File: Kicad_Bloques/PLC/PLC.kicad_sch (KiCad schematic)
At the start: 3 parts, among them J1 Conn_01x18_Socket, J2 Conn_01x18_Socket, U1 ESP32-S3-WROOM-1

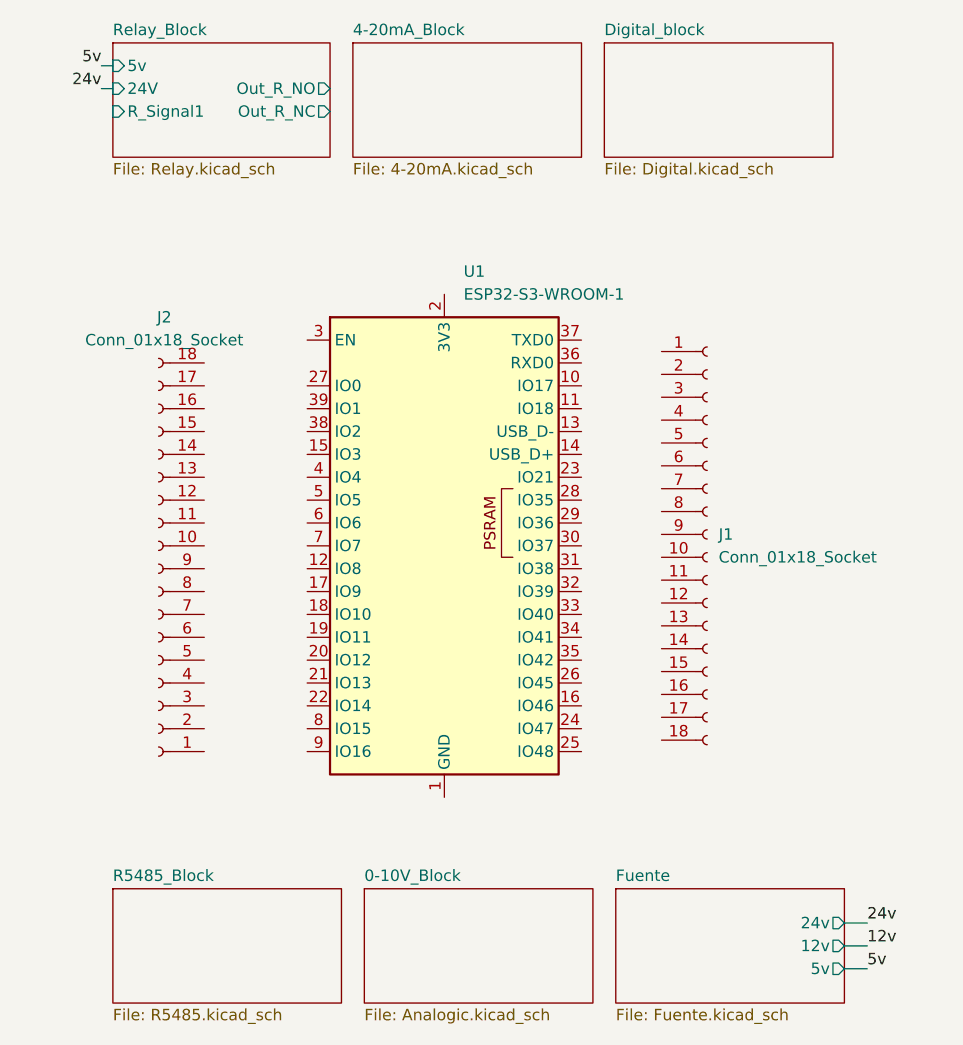
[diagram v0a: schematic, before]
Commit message: Actualizacion Bloques e Investigacion
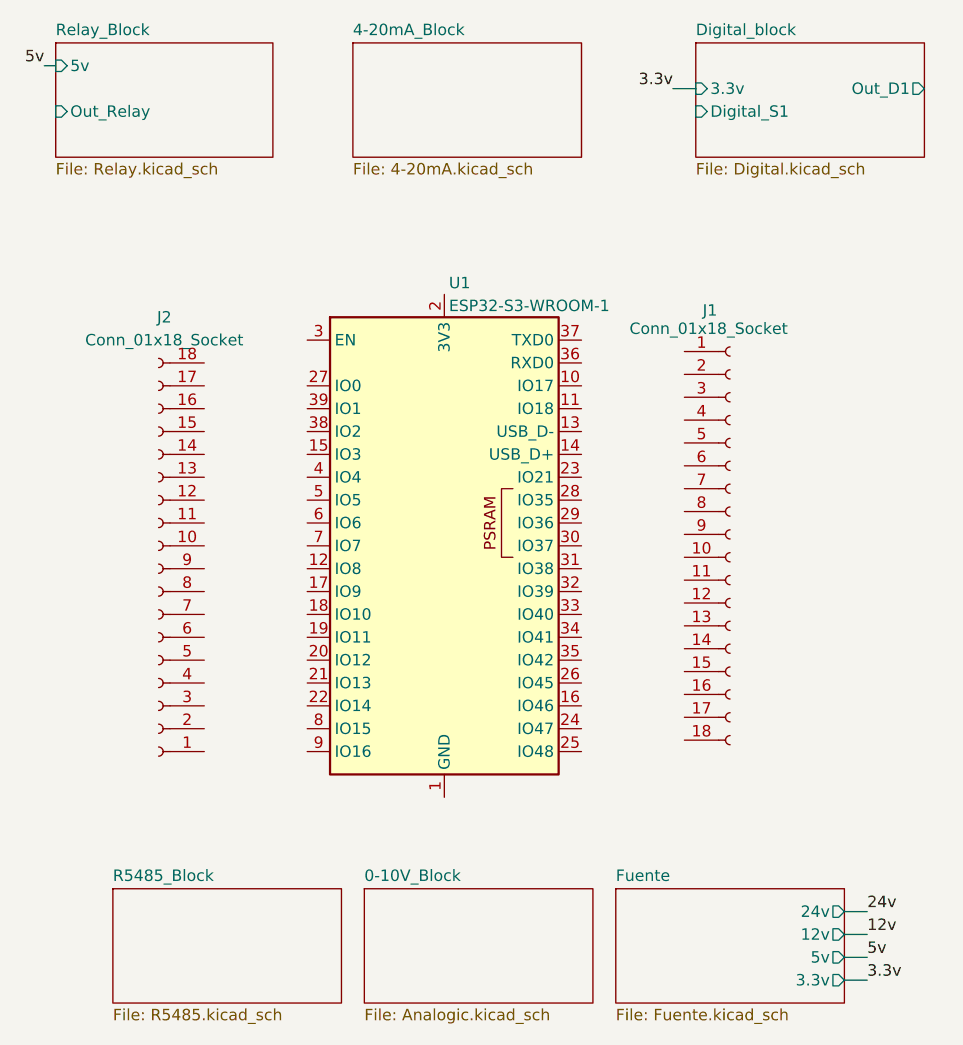
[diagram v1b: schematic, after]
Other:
- sheet Digital_block ports: added 3.3v, Digital_S1, Out_D1; removed none
- sheet Fuente ports: added 3.3v; removed none
- sheet Relay_Block ports: added Out_Relay; removed 24V, Out_R_NC, Out_R_NO, R_Signal1
- moved on the sheet: J1
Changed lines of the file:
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@@
 	(wire
 		(pts
-			(xy 163.83 139.7) (xy 166.37 139.7)
+			(xy 163.83 138.43) (xy 166.37 138.43)
 		)
 		(stroke
@@
 	(wire
 		(pts
-			(xy 81.28 41.91) (xy 82.55 41.91)
+			(xy 163.83 135.89) (xy 166.37 135.89)
 		)
 		(stroke
@@
 	(wire
 		(pts
-			(xy 163.83 137.16) (xy 166.37 137.16)
+			(xy 74.93 39.37) (xy 76.2 39.37)
 		)
 		(stroke
@@
 	(wire
 		(pts
-			(xy 81.28 39.37) (xy 82.55 39.37)
+			(xy 163.83 140.97) (xy 166.37 140.97)
 		)
 		(stroke
@@
 	(wire
 		(pts
-			(xy 163.83 134.62) (xy 166.37 134.62)
+			(xy 163.83 133.35) (xy 166.37 133.35)
 		)
 		(stroke
@@
 		)
 	)
+	(wire
+		(pts
+			(xy 144.78 41.91) (xy 147.32 41.91)
+		)
+		(stroke
+			(width 0)
+			(type default)
+		)
+	)
 	(label "12v"
-		(at 166.37 137.16 0)
+		(at 166.37 135.89 0)
 		(effects
 			(font
@@
 	)
 	(label "5v"
-		(at 166.37 139.7 0)
+		(at 166.37 138.43 0)
 		(effects
 			(font
@@
 	)
 	(label "24v"
-		(at 166.37 134.62 0)
+		(at 166.37 133.35 0)
 		(effects
 			(font
@@
 		)
 	)
-	(label "24v"
-		(at 81.28 41.91 180)
+	(label "3.3v"
+		(at 144.78 41.91 180)
 		(effects
 			(font
 				(size 1.27 1.27)
+				(thickness 0.1588)
 			)
 			(justify right bottom)
@@
 	)
 	(label "5v"
-		(at 81.28 39.37 180)
+		(at 74.93 39.37 180)
 		(effects
 			(font
@@
 			)
 			(justify right bottom)
+		)
+	)
+	(label "3.3v"
+		(at 166.37 140.97 0)
+		(effects
+			(font
+				(size 1.27 1.27)
+				(thickness 0.1588)
+			)
+			(justify left bottom)
 		)
 	)
@@
 		(on_board yes)
 		(dnp no)
-		(fields_autoplaced yes)
 		(property "Reference" "U1"
-			(at 121.5233 62.23 0)
+			(at 119.888 63.5 0)
 			(effects
 				(font
@@
 		)
 		(property "Value" "ESP32-S3-WROOM-1"
-			(at 121.5233 64.77 0)
+			(at 119.888 66.04 0)
 			(effects
 				(font
@@
 	(symbol
 		(lib_id "Connector:Conn_01x18_Socket")
-		(at 148.59 91.44 0)
+		(at 151.13 91.44 0)
 		(unit 1)
 		(exclude_from_sim no)
@@
 		(on_board yes)
 		(dnp no)
-		(fields_autoplaced yes)
 		(property "Reference" "J1"
-			(at 149.86 91.4399 0)
+			(at 148.082 66.548 0)
 			(effects
 				(font
@@
 		)
 		(property "Value" "Conn_01x18_Socket"
-			(at 149.86 93.9799 0)
+			(at 139.954 68.58 0)
 			(effects
 				(font
@@
 		)
 		(property "Footprint" ""
-			(at 148.59 91.44 0)
+			(at 151.13 91.44 0)
 			(effects
 				(font
@@
 		)
 		(property "Datasheet" "~"
-			(at 148.59 91.44 0)
+			(at 151.13 91.44 0)
 			(effects
 				(font
@@
 		)
 		(property "Description" "Generic connector, single row, 01x18, script generated"
-			(at 148.59 91.44 0)
+			(at 151.13 91.44 0)
 			(effects
 				(font
@@
 		)
 		(pin "24v" output
-			(at 163.83 134.62 0)
+			(at 163.83 133.35 0)
 			(effects
 				(font
@@
 		)
 		(pin "5v" output
-			(at 163.83 139.7 0)
+			(at 163.83 138.43 0)
 			(effects
 				(font
@@
 		)
 		(pin "12v" output
-			(at 163.83 137.16 0)
+			(at 163.83 135.89 0)
+			(effects
+				(font
+					(size 1.27 1.27)
+				)
+				(justify right)
+			)
+		)
+		(pin "3.3v" output
+			(at 163.83 140.97 0)
 			(effects
 				(font
@@
 	)
 	(sheet
-		(at 137.16 36.83)
+		(at 147.32 36.83)
 		(size 25.4 12.7)
 		(exclude_from_sim no)
@@
 		)
 		(property "Sheetname" "Digital_block"
-			(at 137.16 36.1184 0)
+			(at 147.32 36.1184 0)
 			(effects
 				(font
@@
 		)
 		(property "Sheetfile" "Digital.kicad_sch"
-			(at 137.16 50.1146 0)
+			(at 147.32 50.1146 0)
 			(effects
 				(font
@@
 				)
 				(justify left top)
+			)
+		)
+		(pin "Out_D1" output
+			(at 172.72 41.91 0)
+			(effects
+				(font
+					(size 1.27 1.27)
+				)
+				(justify right)
+			)
+		)
+		(pin "Digital_S1" input
+			(at 147.32 44.45 180)
+			(effects
+				(font
+					(size 1.27 1.27)
+				)
+				(justify left)
+			)
+		)
+		(pin "3.3v" input
+			(at 147.32 41.91 180)
+			(effects
+				(font
+					(size 1.27 1.27)
+				)
+				(justify left)
 			)
 		)
@@
 	)
 	(sheet
-		(at 82.55 36.83)
+		(at 76.2 36.83)
 		(size 24.13 12.7)
 		(exclude_from_sim no)
@@
 		)
 		(property "Sheetname" "Relay_Block"
-			(at 82.55 36.1184 0)
+			(at 76.2 36.1184 0)
 			(effects
 				(font
@@
 		)
 		(property "Sheetfile" "Relay.kicad_sch"
-			(at 82.55 50.1146 0)
+			(at 76.2 50.1146 0)
 			(effects
 				(font
@@
 			)
 		)
-		(pin "Out_R_NO" output
-			(at 106.68 41.91 0)
-			(effects
-				(font
-					(size 1.27 1.27)
-				)
-				(justify right)
-			)
-		)
-		(pin "Out_R_NC" output
-			(at 106.68 44.45 0)
-			(effects
-				(font
-					(size 1.27 1.27)
-				)
-				(justify right)
-			)
-		)
-		(pin "R_Signal1" input
-			(at 82.55 44.45 180)
+		(pin "5v" input
+			(at 76.2 39.37 180)
 			(effects
 				(font
@@
 			)
 		)
-		(pin "5v" input
-			(at 82.55 39.37 180)
-			(effects
-				(font
-					(size 1.27 1.27)
-				)
-				(justify left)
-			)
-		)
-		(pin "24V" input
-			(at 82.55 41.91 180)
-			(effects
-				(font
+		(pin "Out_Relay" input
+			(at 76.2 44.45 180)
+			(effects
+				(font
